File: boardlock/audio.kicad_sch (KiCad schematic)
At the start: 16 parts, among them J3 Micro_SD_Card_Det1, U7 MAX98357AETE+T

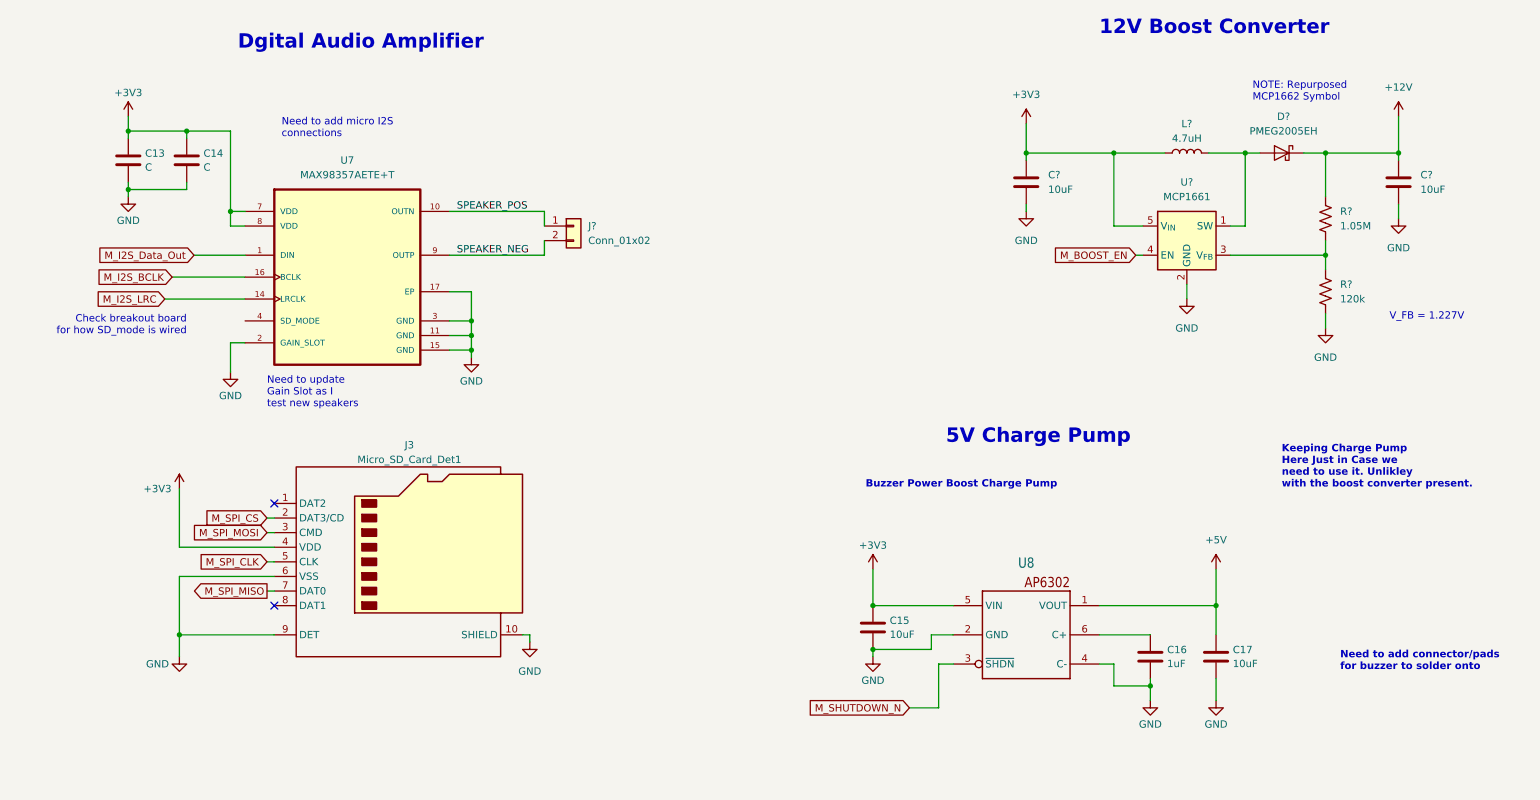
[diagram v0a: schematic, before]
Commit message: saving
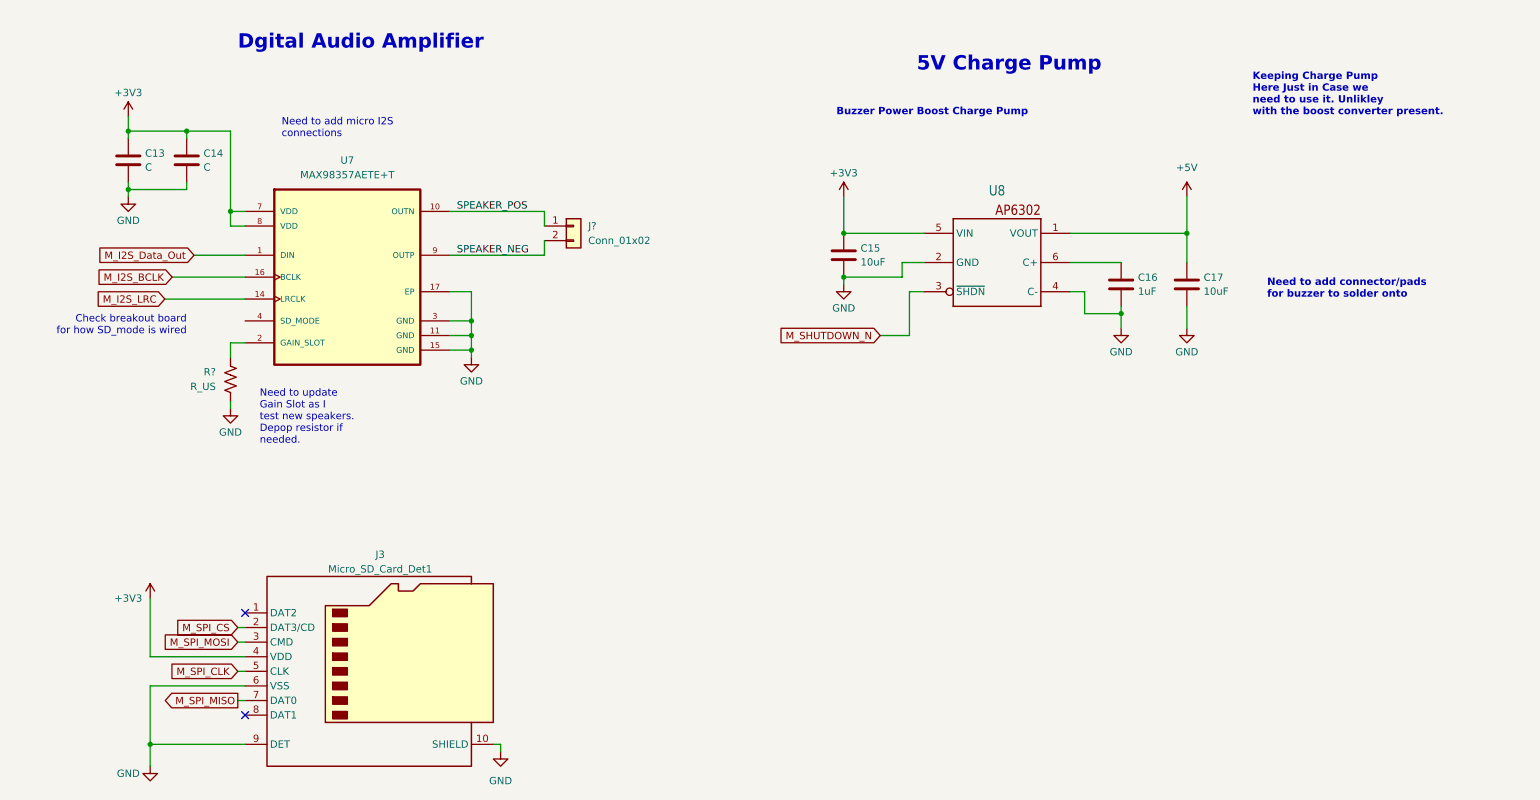
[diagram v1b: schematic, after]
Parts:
- removed C? (x2): 10uF, symbol Device:C
- removed D?: PMEG2005EH, Diode_SMD:D_SOD-123F, symbol Diode:PMEG2005EH
- removed L?: 4.7uH, symbol Device:L
- removed R?: 1.05M, symbol Device:R_US
- removed R?: 120k, symbol Device:R_US
- removed U?: MCP1661, Package_TO_SOT_SMD:SOT-23-5, symbol Driver_LED:MCP1662-xOT
- added R?: R_US, symbol Device:R_US
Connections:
- net GND: now also R?.2; no longer U7.2 (GAIN_SLOT)
- new net: R?.1, U7.2 (GAIN_SLOT)
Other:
- note added: "Need to update Gain Slot as I test new speakers. Depop resistor if needed."
- note removed: "12V Boost Converter"
- note removed: "NOTE: Repurposed MCP1662 Symbol"
- note removed: "Need to update Gain Slot as I test new speakers"
- note removed: "V_FB = 1.227V"
- moved on the sheet: C15, C16, C17, J3, U8
